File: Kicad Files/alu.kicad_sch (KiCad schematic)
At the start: 27 parts, among them U40 SST39SF040, U41 SST39SF040, U42 74LS173

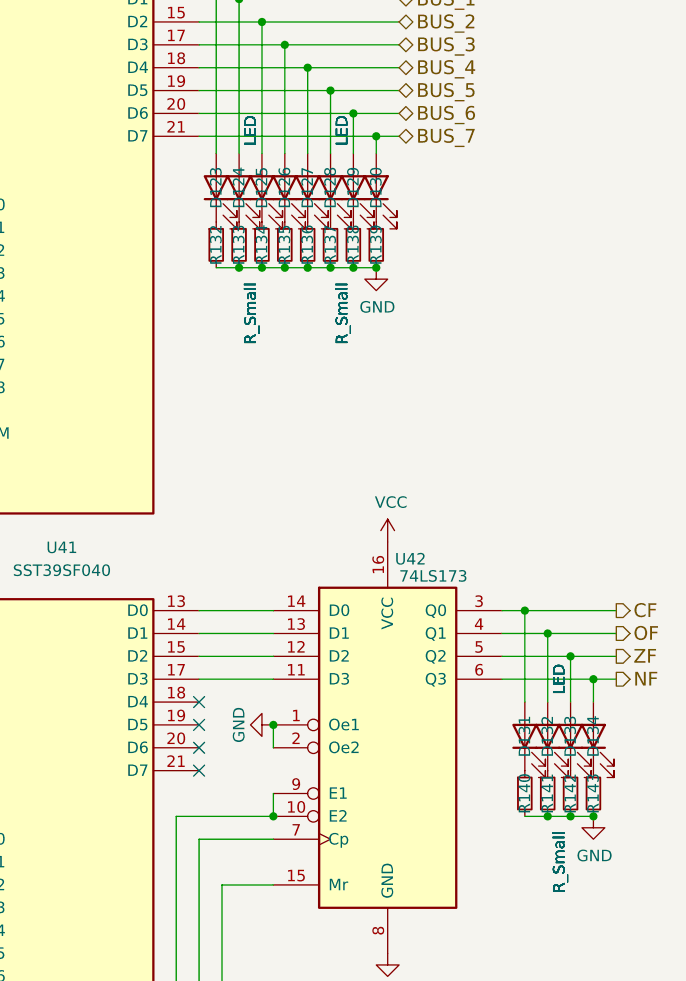
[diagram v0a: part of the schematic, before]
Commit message: updated library
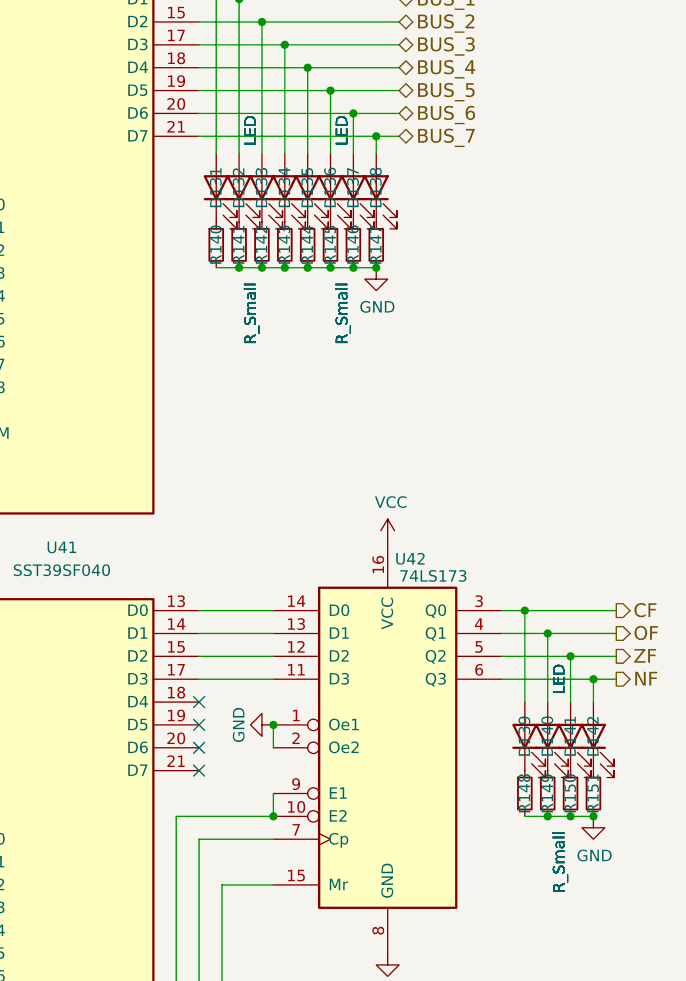
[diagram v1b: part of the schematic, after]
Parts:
- renumbered D123 to D131, D124 to D132, D125 to D133, D126 to D134, D127 to D135, D128 to D136, D129 to D137, D130 to D138, D131 to D139, D132 to D140, D133 to D141, D134 to D142, R132 to R140, R133 to R141, R134 to R142, R135 to R143, R136 to R144, R137 to R145, R138 to R146, R139 to R147, R140 to R148, R141 to R149, R142 to R150, R143 to R151

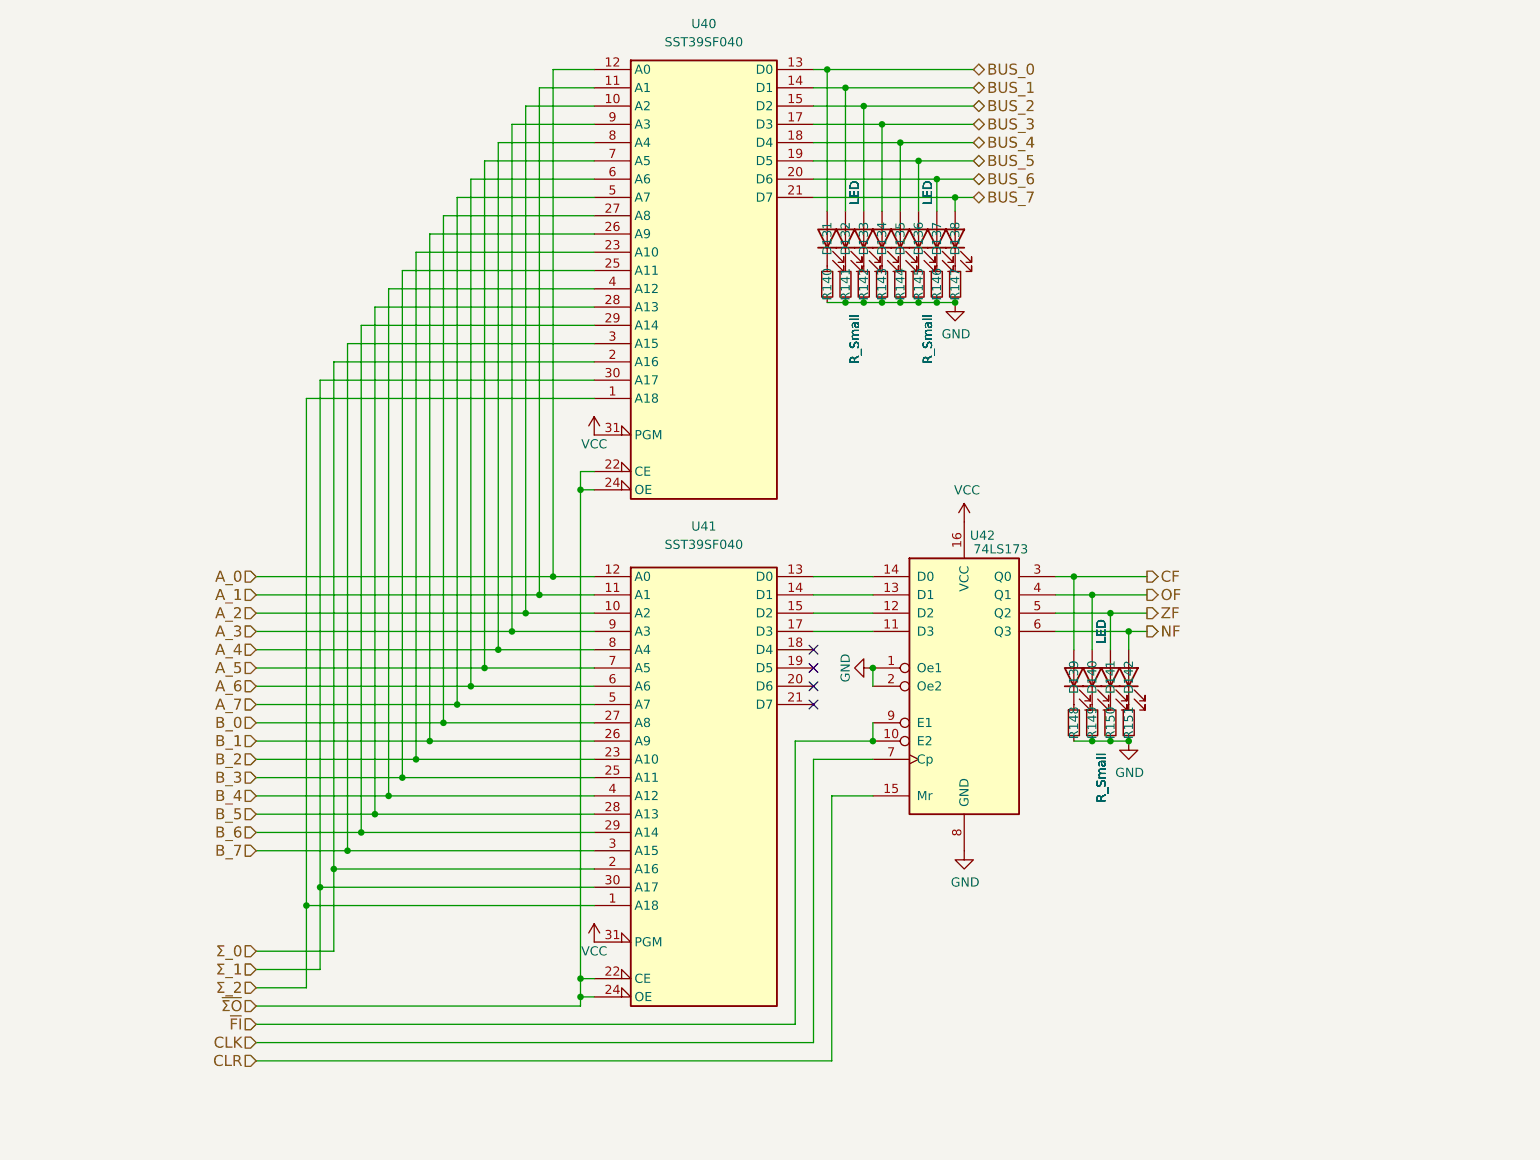
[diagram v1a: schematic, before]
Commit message: im sooo stupiiid
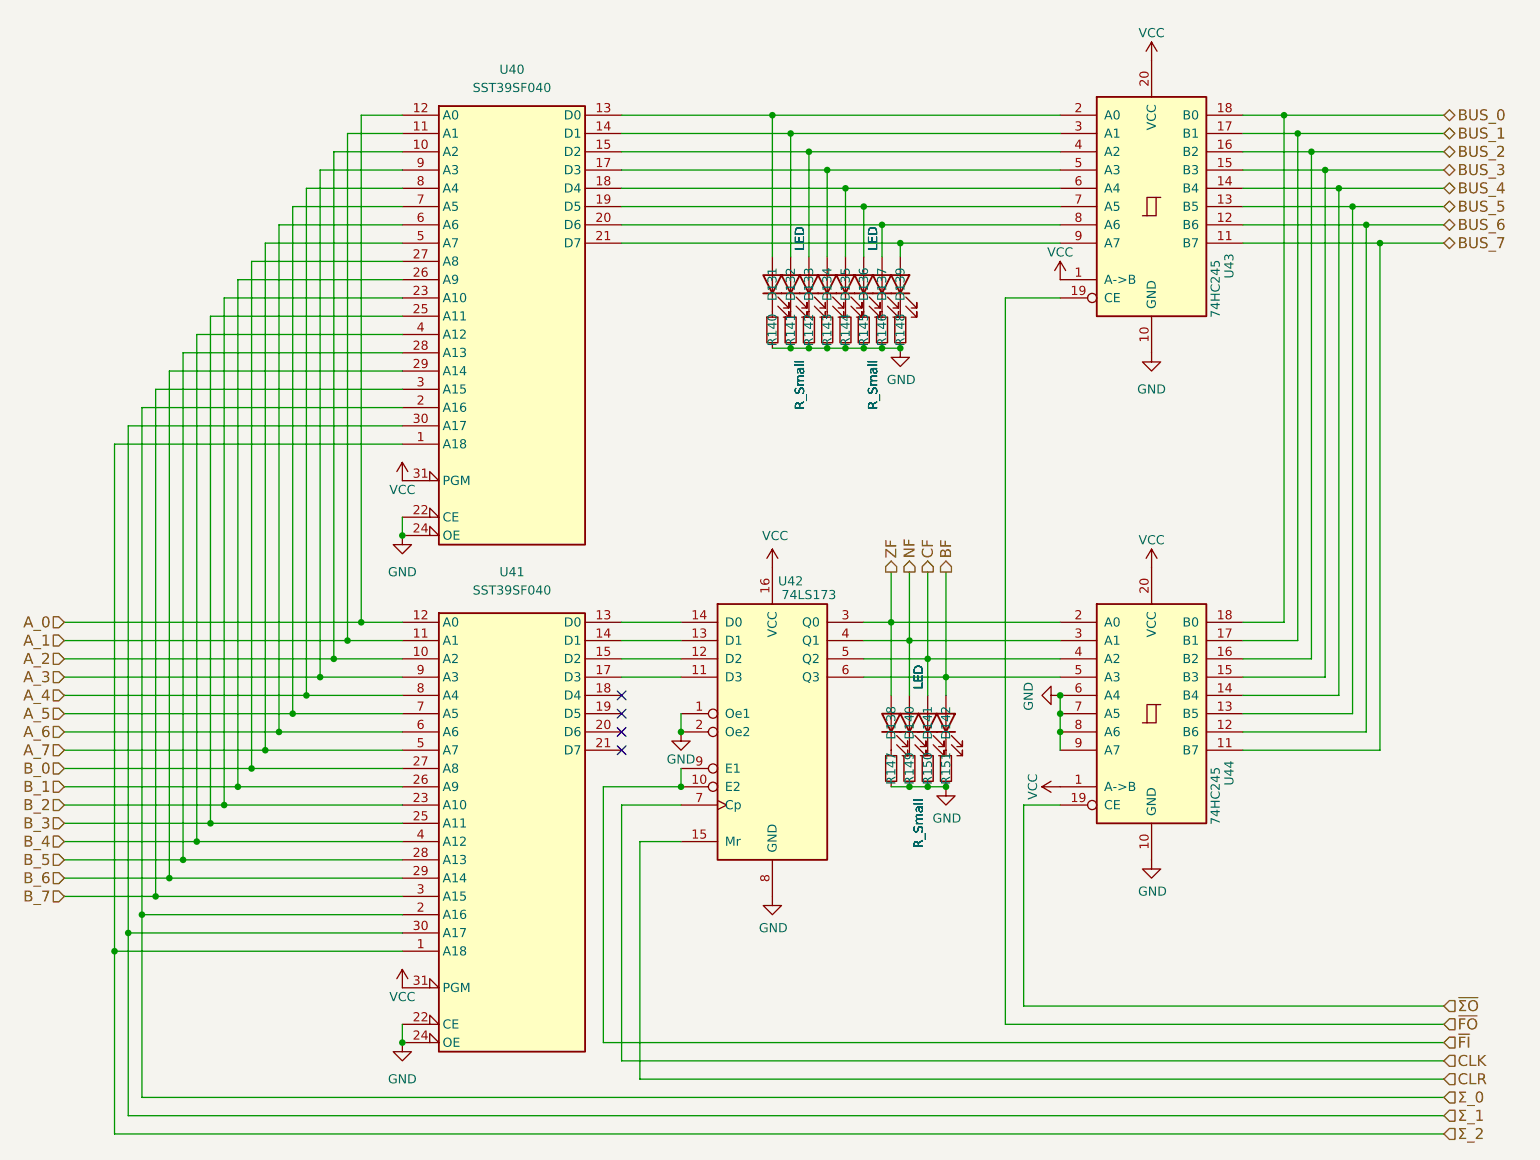
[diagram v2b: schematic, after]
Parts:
- added U43, U44: 74HC245, symbol 74xx:74HC245
- renumbered D139 to D138, D138 to D139, R148 to R147, R147 to R148
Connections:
- net OF is gone; now on net NF: D140.2 (A), U42.4 (Q1)
- net BUS_0: now also U43.18 (B0), U44.18 (B0); no longer D131.2 (A), U40.13 (D0)
- net BUS_1: now also U43.17 (B1), U44.17 (B1); no longer D132.2 (A), U40.14 (D1)
- net BUS_2: now also U43.16 (B2), U44.16 (B2); no longer D133.2 (A), U40.15 (D2)
- net BUS_3: now also U43.15 (B3), U44.15 (B3); no longer D134.2 (A), U40.17 (D3)
- net BUS_4: now also U43.14 (B4), U44.14 (B4); no longer D135.2 (A), U40.18 (D4)
- net BUS_5: now also U43.13 (B5), U44.13 (B5); no longer D136.2 (A), U40.19 (D5)
- net BUS_6: now also U43.12 (B6), U44.12 (B6); no longer D137.2 (A), U40.20 (D6)
- net BUS_7: now also U43.11 (B7), U44.11 (B7); no longer D139.2 (A), U40.21 (D7)
- net CF: now also D141.2 (A), U42.5 (Q2), U44.4 (A2); no longer D138.2 (A), U42.3 (Q0)
- net GND: now also U40.22 (CE), U40.24 (OE), U41.22 (CE), U41.24 (OE), U43.10 (GND), U44.10 (GND), U44.6 (A4), U44.7 (A5), U44.8 (A6), U44.9 (A7)
- net NF: now also U44.3 (A1); no longer D142.2 (A), U42.6 (Q3)
- net VCC: now also U43.1 (A->B), U43.20 (VCC), U44.1 (A->B), U44.20 (VCC)
- net ZF: now also D138.2 (A), U42.3 (Q0), U44.2 (A0); no longer D141.2 (A), U42.5 (Q2)
- net ~{ΣO}: now also U44.19 (CE); no longer U40.22 (CE), U40.24 (OE), U41.22 (CE), U41.24 (OE)
- new net: D133.2 (A), U40.15 (D2), U43.4 (A2)
- new net: D136.2 (A), U40.19 (D5), U43.7 (A5)
- new net: D131.2 (A), U40.13 (D0), U43.2 (A0)
- new net: D134.2 (A), U40.17 (D3), U43.5 (A3)
- new net: D139.2 (A), U40.21 (D7), U43.9 (A7)
- new net: D132.2 (A), U40.14 (D1), U43.3 (A1)
- new net: D135.2 (A), U40.18 (D4), U43.6 (A4)
- new net: D137.2 (A), U40.20 (D6), U43.8 (A6)
- new net BF: D142.2 (A), U42.6 (Q3), U44.5 (A3)
- new net ~{FO}: U43.19 (CE)
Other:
- moved on the sheet: D131, D132, D133, D134, D135, D136, D137, D138, D139, D140, D141, D142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
